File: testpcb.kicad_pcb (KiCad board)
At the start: 2 copper layers, 52 parts, among them SW1 SW_Push, U1 ATmega16U4-AU, Y1 16MHz

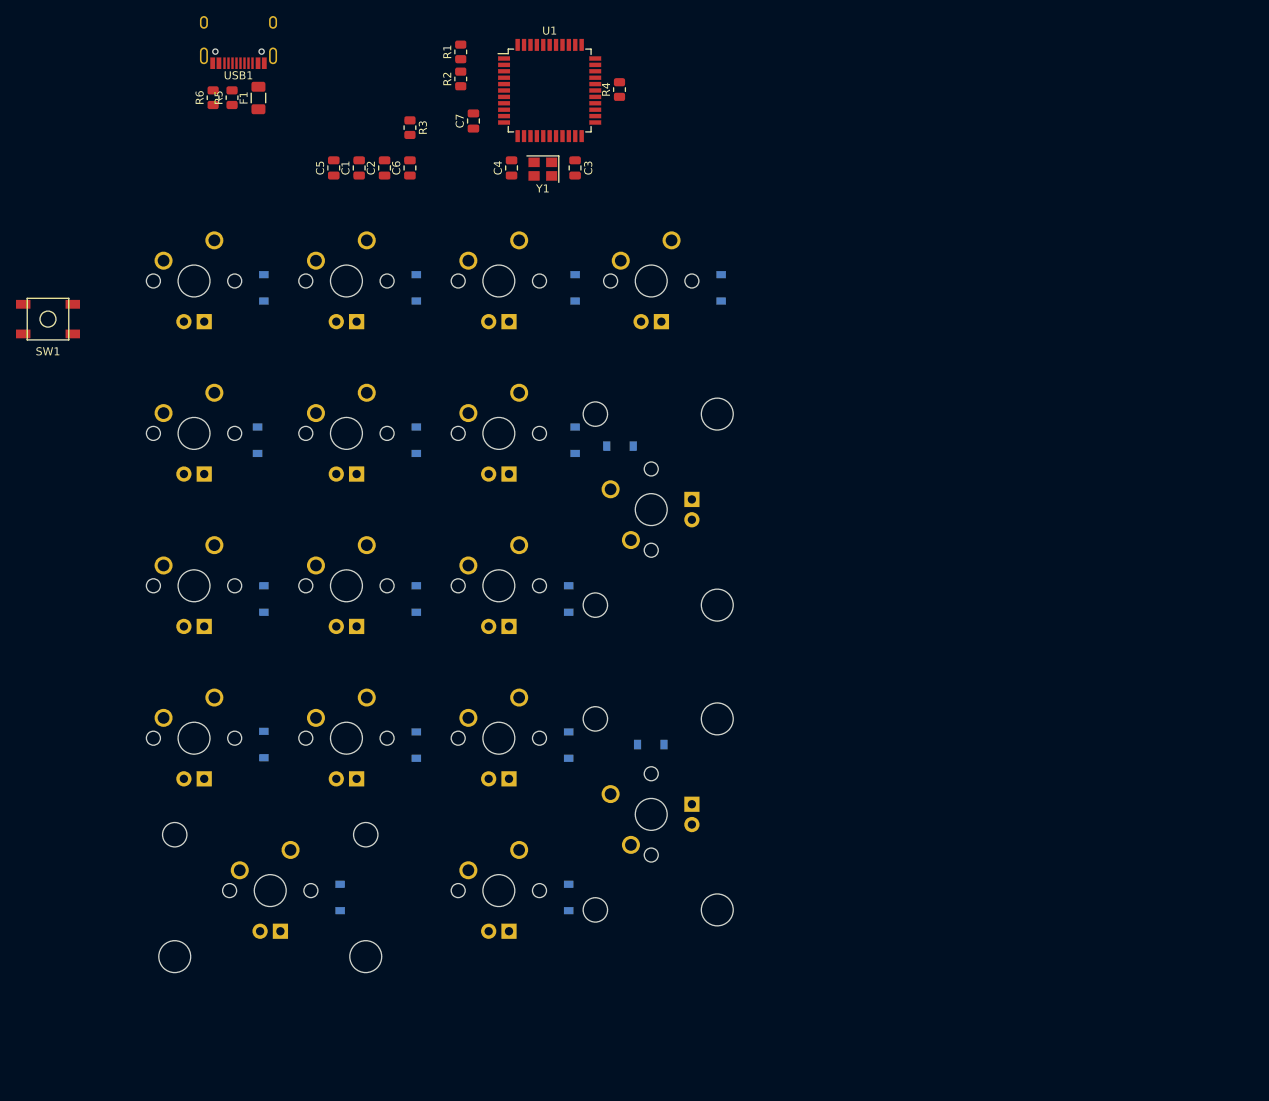
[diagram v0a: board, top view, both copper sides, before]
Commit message: DONE
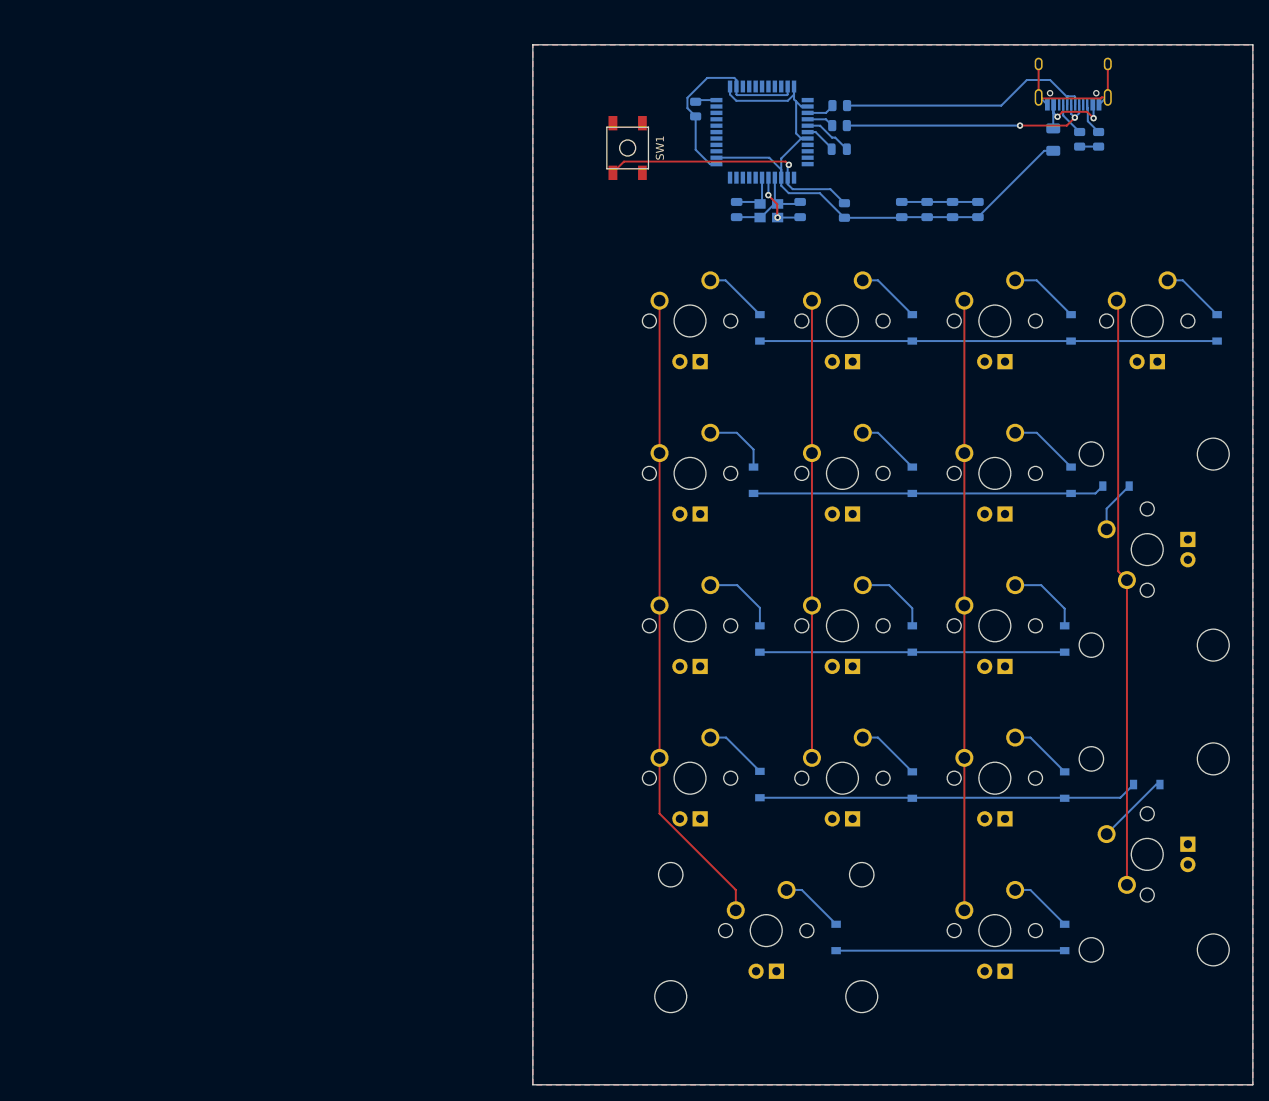
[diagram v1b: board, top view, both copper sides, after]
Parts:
- C1, C2, C3, C4, C5, C6, C7, F1, R1, R2, R3, R4, R5, R6, U1, USB1, Y1: moved to B.Cu
- moved R6 110.8 mm to (360.7, -8.19)
- moved R5 106.1 mm to (358.4, -8.19)
- moved USB1 104.5 mm to (357.5, -20.2), turned to 0 degrees
- moved F1 99.5 mm to (355.1, -8.15)
- moved C5 80.7 mm to (345.6, 0.59)
- moved SW1 75.5 mm to (301.9, -7.10), turned to 90 degrees
- moved C1 74.4 mm to (342.5, 0.59)
- moved C2 68.0 mm to (339.3, 0.59)
- moved D1 62.2 mm to (318.4, 15.4)
- moved D10 62.2 mm to (357.3, 15.4)
- moved D11 62.2 mm to (357.3, 34.4)
- moved D12 62.2 mm to (356.5, 54.3)
- moved D13 62.2 mm to (356.5, 72.5)
- moved D14 62.2 mm to (356.5, 91.6)
- moved D15 62.2 mm to (375.5, 15.4)
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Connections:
- USB1 pad 11: Net-(USB1-Pad11) -> VCC
- USB1 pad 12: Net-(USB1-Pad12) -> GND
- USB1 pad 13: Net-(USB1-Pad13) -> GND
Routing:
- net COL0: track 0.00 -> 80.1 mm
- net GND: track 0.00 -> 77.9 mm
- net COL2: track 0.00 -> 76.2 mm
- net +5V: track 0.00 -> 75.8 mm
- net COL3: track 0.00 -> 73.6 mm
- net COL1: track 0.00 -> 57.2 mm
- net ROW0: track 0.00 -> 57.1 mm
- net ROW3: track 0.00 -> 47.4 mm
- net ROW1: track 0.00 -> 44.0 mm
- net ROW2: track 0.00 -> 38.1 mm
- net Net-(R3-Pad2): track 0.00 -> 33.3 mm, vias 0 -> 1
- net D-: track 0.00 -> 32.7 mm
- net D+: track 0.00 -> 32.5 mm, vias 0 -> 2
- net ROW4: track 0.00 -> 28.6 mm
- net VCC: track 0.00 -> 11.5 mm, vias 0 -> 2
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- added copper zone on B.Cu, net GND
- added copper zone on F.Cu, net GND
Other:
- board outline added: 90 x 130 mm
